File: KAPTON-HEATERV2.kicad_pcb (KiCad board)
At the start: 2 copper layers, 90 x 76 mm, 33 parts, among them J1 XT60PW-M, J2 XT60PW-M, J3 1985276, J4 1985218, J5 10090926-P154XLF, K1 1-1393210-8, Q1 AO3400A, U1 TC4427ACOA, U2 INA181

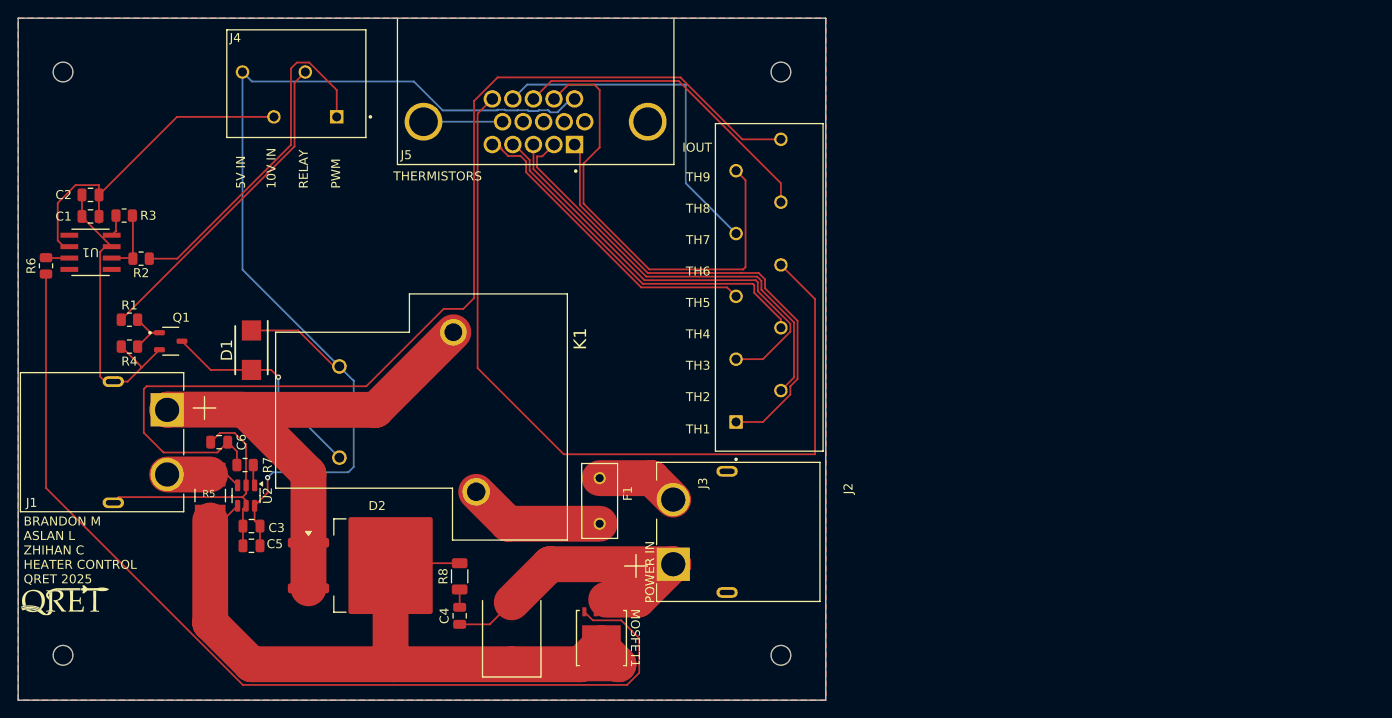
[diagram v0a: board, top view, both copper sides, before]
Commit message: June 26 New Traces
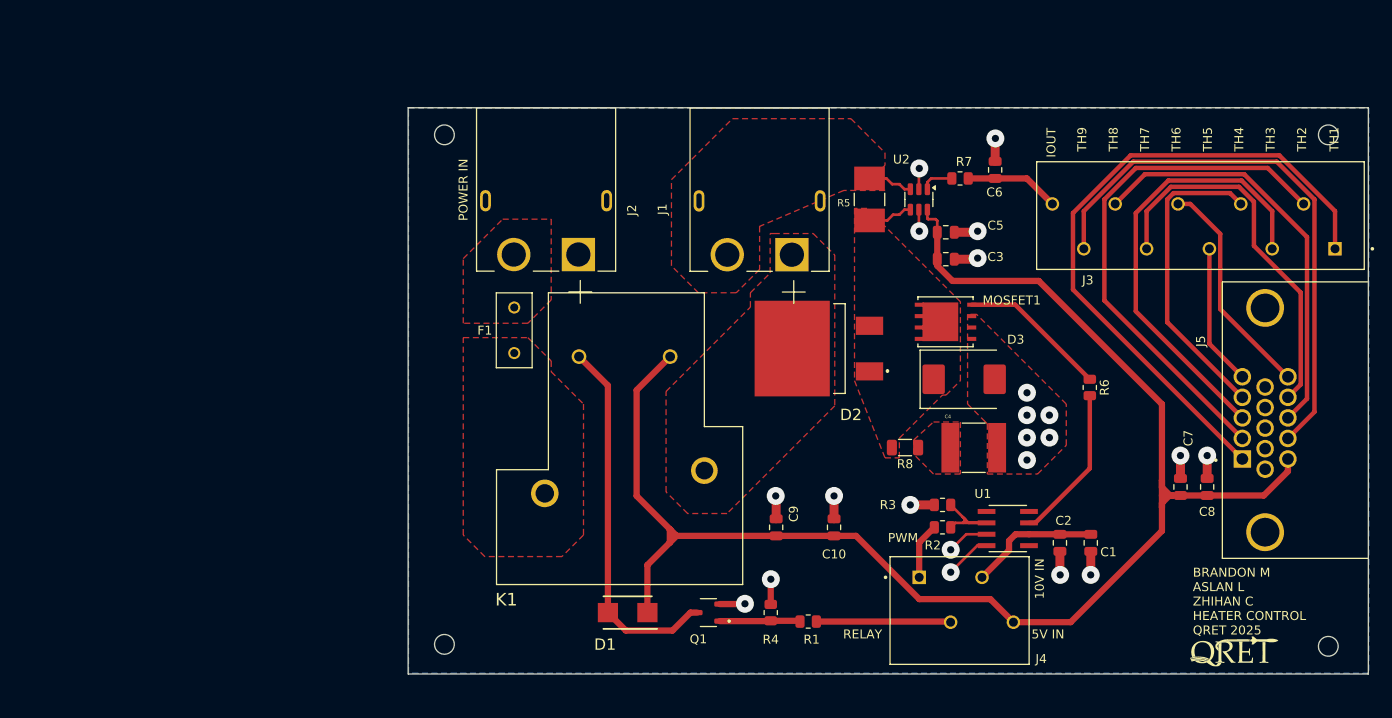
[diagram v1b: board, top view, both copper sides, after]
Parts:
- added C10: C4.7uf, Capacitor_SMD:C_0805_2012Metric, F.Cu at (140.9, 115.7)
- added C7: C4.7uf, Capacitor_SMD:C_0805_2012Metric, F.Cu at (179.5, 111.2)
- added C8: C0.1uf, Capacitor_SMD:C_0805_2012Metric, F.Cu at (182.5, 111.2)
- added C9: C0.1uf, Capacitor_SMD:C_0805_2012Metric, F.Cu at (134.5, 115.7)
- C4: footprint Capacitor_SMD:C_0805_2012Metric -> KCM55LR71J475KH01K:CAPC6153X300N
- D2: value V20DM100C-M3/I -> V20DM100C-M3_I; footprint Package_TO_SOT_SMD:TO-263-2 -> LIB_V20DM100C-M3_I:V40DL45BPM3I
- moved G*** 130.4 mm to (185.5, 129.5)
- moved C1 117.3 mm to (169.5, 117.5), turned to -90 degrees
- moved R6 117.1 mm to (169.4, 100.2), turned to -90 degrees
- moved C2 114.8 mm to (166.1, 117.5), turned to -90 degrees
- moved U1 106.8 mm to (160.3, 115.9), turned to 0 degrees
- moved R3 96.7 mm to (153.0, 113.2)
- moved J4 94.4 mm to (154.9, 125.0), turned to 0 degrees
- moved R2 94.2 mm to (153.0, 115.7), turned to 0 degrees
- moved C6 91.6 mm to (158.9, 75.9), turned to 90 degrees
- moved J5 87.8 mm to (189.0, 103.8), turned to 90 degrees
- moved R7 85.8 mm to (155.0, 76.9), turned to 180 degrees
- moved C5 84.9 mm to (153.4, 82.9), turned to 180 degrees
- moved C3 82.9 mm to (153.4, 85.9), turned to 180 degrees
- moved R1 82.8 mm to (138.0, 126.2), turned to 180 degrees
- moved U2 81.9 mm to (150.4, 79.2)
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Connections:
- D2 pad 1: /24V -> HEATER OUT
- J1 pad S1: GND -> (no net)
- J1 pad S2: GND -> (no net)
- J2 pad S1: GND -> (no net)
- J2 pad S2: GND -> (no net)
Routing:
- net Current Vout: track 119.7 -> 10.6 mm
- net Net-(MOSFET1-Pad4): track 110.8 -> 16.6 mm
- net HEATER OUT: track 87.0 -> 5.05 mm
- net TH6: track 94.9 -> 25.1 mm
- net GND: track 112.4 -> 46.9 mm, vias 0 -> 22
- net /24V: track 58.1 -> 0.00 mm
- net 5V: track 118.7 -> 169.9 mm, vias 1 -> 0
- net PWM: track 39.2 -> 6.27 mm
- net 10V: track 39.2 -> 14.7 mm
- net RELAY: track 36.1 -> 15.0 mm
- net TH1: track 53.1 -> 73.9 mm
- net TH5: track 35.0 -> 15.8 mm
- net Net-(D1-A): track 24.2 -> 41.5 mm, vias 1 -> 0
- net Net-(F1-Pad2): track 15.2 -> 0.00 mm
- net 10V PWM: track 2.56 -> 17.4 mm
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- added copper zone on F.Cu, net /24V
- added copper zone on F.Cu, net HEATER OUT
- added copper zone on F.Cu, net Net-(C4-Pad1)
- added copper zone on F.Cu, net Net-(F1-Pad2)
- added copper zone on F.Cu, net Net-(J2--)
- added copper zone on F.Cu, net SHUNT HIGH
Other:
- board size 90 x 76 mm -> 107 x 63.1 mm
- board text added: "C0.1uf"
- board text added: "C4.7uf"
- board text added: "D3"
- board text added: "R5"
- board text removed: "THERMISTORS"
